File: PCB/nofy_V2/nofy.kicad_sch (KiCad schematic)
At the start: 153 parts, among them J18 PIn1x4, J21 PIn1x4, J32 PIn1x4, J33 PIn1x4, SW1 SW_SPDT, SW10 SW_PUSH, SW11 SW_PUSH, SW12 SW_PUSH, SW13 SW_PUSH, SW14 SW_PUSH, SW15 SW_PUSH, SW16 SW_PUSH, SW17 SW_PUSH, SW18 SW_PUSH, SW19 SW_PUSH, SW2 SW_SPDT, SW20 SW_PUSH, SW21 SW_PUSH, SW22 SW_PUSH, SW23 SW_PUSH, SW24 SW_PUSH, SW25 SW_PUSH, SW26 SW_PUSH, SW27 SW_PUSH, SW28 SW_PUSH, SW29 SW_PUSH, SW3 RotaryEncoder, SW30 SW_PUSH, SW31 SW_PUSH, SW32 SW_PUSH, SW33 SW_PUSH, SW34 SW_PUSH, SW35 SW_PUSH, SW36 SW_PUSH, SW37 SW_PUSH, SW38 SW_PUSH, SW39 SW_PUSH, SW4 RotaryEncoder, SW40 SW_PUSH, SW41 SW_PUSH, SW42 SW_PUSH, SW43 SW_PUSH, SW44 SW_PUSH, SW45 SW_PUSH, SW46 SW_PUSH, SW47 SW_PUSH, SW48 SW_PUSH, SW49 SW_PUSH, SW5 SW_PUSH, SW50 SW_PUSH, SW51 SW_PUSH, SW52 SW_PUSH, SW53 SW_PUSH, SW54 SW_PUSH, SW55 SW_PUSH, SW6 SW_PUSH, SW7 SW_PUSH, SW8 SW_PUSH, SW9 SW_PUSH

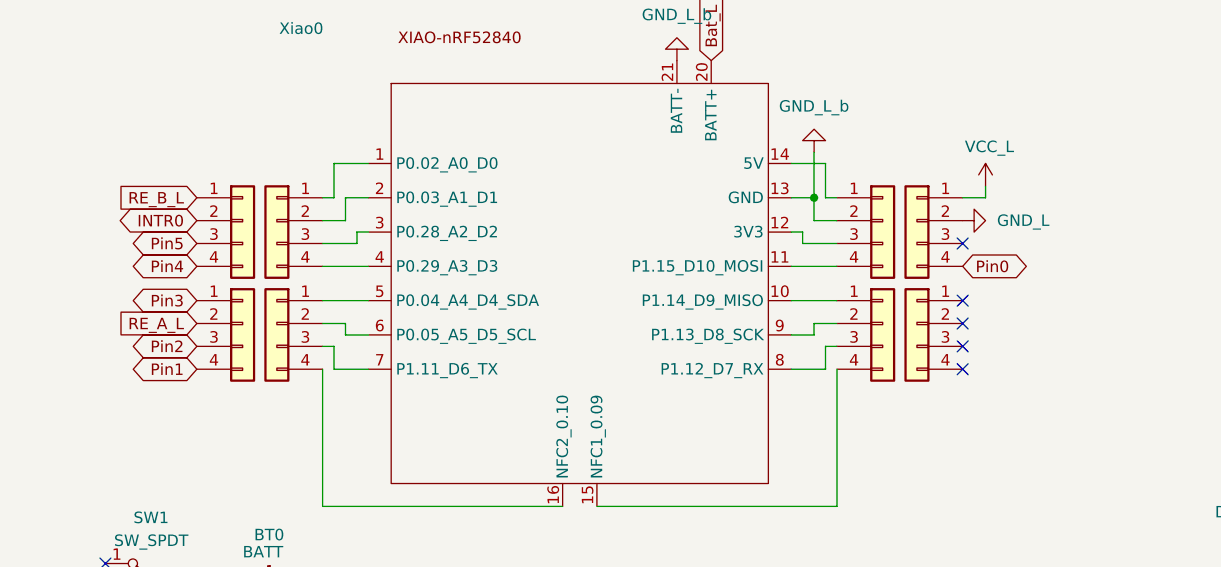
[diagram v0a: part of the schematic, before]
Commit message: PCB
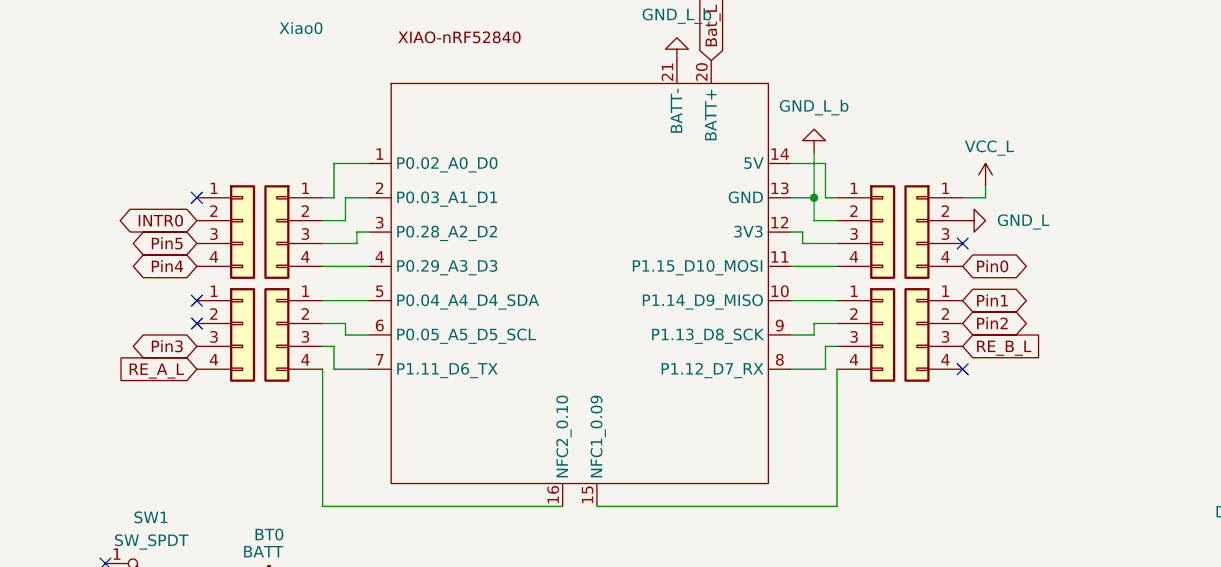
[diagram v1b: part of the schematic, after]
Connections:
- net Pin1: now also Con_L_6.1 (Pin_1); no longer Con_L_2.4 (Pin_4)
- net Pin2: now also Con_L_6.2 (Pin_2); no longer Con_L_2.3 (Pin_3)
- net Pin3: now also Con_L_2.3 (Pin_3); no longer Con_L_2.1 (Pin_1)
- net RE_A_L: now also Con_L_2.4 (Pin_4); no longer Con_L_2.2 (Pin_2)
- net RE_B_L: now also Con_L_6.3 (Pin_3); no longer Con_L_0.1 (Pin_1)
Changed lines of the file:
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@@
 	)
 	(no_connect
-		(at 114.3 55.88)
-	)
-	(no_connect
 		(at 19.05 82.55)
 	)
@@
 	)
 	(no_connect
-		(at 114.3 53.34)
+		(at 29.21 55.88)
 	)
 	(no_connect
-		(at 114.3 58.42)
+		(at 29.21 41.91)
+	)
+	(no_connect
+		(at 29.21 53.34)
 	)
 	(wire
@@
 		)
 	)
+	(global_label "Pin2"
+		(shape bidirectional)
+		(at 114.3 55.88 0)
+		(fields_autoplaced yes)
+		(effects
+			(font
+				(size 1.27 1.27)
+			)
+			(justify left)
+		)
+		(property "Intersheetrefs" "${INTERSHEET_REFS}"
+			(at 122.6298 55.88 0)
+			(effects
+				(font
+					(size 1.27 1.27)
+				)
+				(justify left)
+				(hide yes)
+			)
+		)
+	)
 	(global_label "Pin4"
 		(shape bidirectional)
@@
 		)
 	)
-	(global_label "Pin2"
-		(shape bidirectional)
-		(at 29.21 58.42 180)
-		(fields_autoplaced yes)
-		(effects
-			(font
-				(size 1.27 1.27)
-			)
-			(justify right)
-		)
-		(property "Intersheetrefs" "${INTERSHEET_REFS}"
-			(at 20.8802 58.42 0)
-			(effects
-				(font
-					(size 1.27 1.27)
-				)
-				(justify right)
-				(hide yes)
-			)
-		)
-	)
 	(global_label "RE_B_R"
 		(shape input)
@@
 		)
 	)
-	(global_label "Pin1"
-		(shape bidirectional)
-		(at 29.21 60.96 180)
+	(global_label "RE_B_L"
+		(shape input)
+		(at 114.3 58.42 0)
 		(fields_autoplaced yes)
 		(effects
@@
 				(size 1.27 1.27)
 			)
-			(justify right)
+			(justify left)
 		)
 		(property "Intersheetrefs" "${INTERSHEET_REFS}"
-			(at 20.8802 60.96 0)
+			(at 123.9375 58.42 0)
 			(effects
 				(font
 					(size 1.27 1.27)
 				)
-				(justify right)
+				(justify left)
 				(hide yes)
 			)
@@
 		)
 	)
-	(global_label "RE_A_L"
-		(shape input)
-		(at 29.21 55.88 180)
-		(fields_autoplaced yes)
-		(effects
-			(font
-				(size 1.27 1.27)
-			)
-			(justify right)
-		)
-		(property "Intersheetrefs" "${INTERSHEET_REFS}"
-			(at 19.7539 55.88 0)
-			(effects
-				(font
-					(size 1.27 1.27)
-				)
-				(justify right)
-				(hide yes)
-			)
-		)
-	)
 	(global_label "INTR0"
 		(shape bidirectional)
@@
 		)
 	)
+	(global_label "RE_A_L"
+		(shape input)
+		(at 29.21 60.96 180)
+		(fields_autoplaced yes)
+		(effects
+			(font
+				(size 1.27 1.27)
+			)
+			(justify right)
+		)
+		(property "Intersheetrefs" "${INTERSHEET_REFS}"
+			(at 19.7539 60.96 0)
+			(effects
+				(font
+					(size 1.27 1.27)
+				)
+				(justify right)
+				(hide yes)
+			)
+		)
+	)
 	(global_label "RE_B_L"
 		(shape input)
@@
 		)
 	)
+	(global_label "Pin1"
+		(shape bidirectional)
+		(at 114.3 53.34 0)
+		(fields_autoplaced yes)
+		(effects
+			(font
+				(size 1.27 1.27)
+			)
+			(justify left)
+		)
+		(property "Intersheetrefs" "${INTERSHEET_REFS}"
+			(at 122.6298 53.34 0)
+			(effects
+				(font
+					(size 1.27 1.27)
+				)
+				(justify left)
+				(hide yes)
+			)
+		)
+	)
 	(global_label "SCLK"
 		(shape input)
@@
 		)
 	)
-	(global_label "INTR1"
+	(global_label "Pin3"
 		(shape bidirectional)
-		(at 22.86 200.66 180)
+		(at 29.21 58.42 180)
 		(fields_autoplaced yes)
 		(effects
@@
 		)
 		(property "Intersheetrefs" "${INTERSHEET_REFS}"
-			(at 13.3811 200.66 0)
+			(at 20.8802 58.42 0)
 			(effects
 				(font
@@
 		)
 	)
-	(global_label "Pin3"
+	(global_label "INTR1"
 		(shape bidirectional)
-		(at 29.21 53.34 180)
+		(at 22.86 200.66 180)
 		(fields_autoplaced yes)
 		(effects
@@
 		)
 		(property "Intersheetrefs" "${INTERSHEET_REFS}"
-			(at 20.8802 53.34 0)
+			(at 13.3811 200.66 0)
 			(effects
 				(font
@@
 				(hide yes)
 			)
-		)
-	)
-	(global_label "RE_B_L"
-		(shape input)
-		(at 29.21 41.91 180)
-		(fields_autoplaced yes)
-		(effects
-			(font
-				(size 1.27 1.27)
-			)
-			(justify right)
-		)
-		(property "Intersheetrefs" "${INTERSHEET_REFS}"
-			(at 19.5725 41.91 0)
-			(effects
-				(font
-					(size 1.27 1.27)
-				)
-				(justify right)
-				(hide yes)
-			)

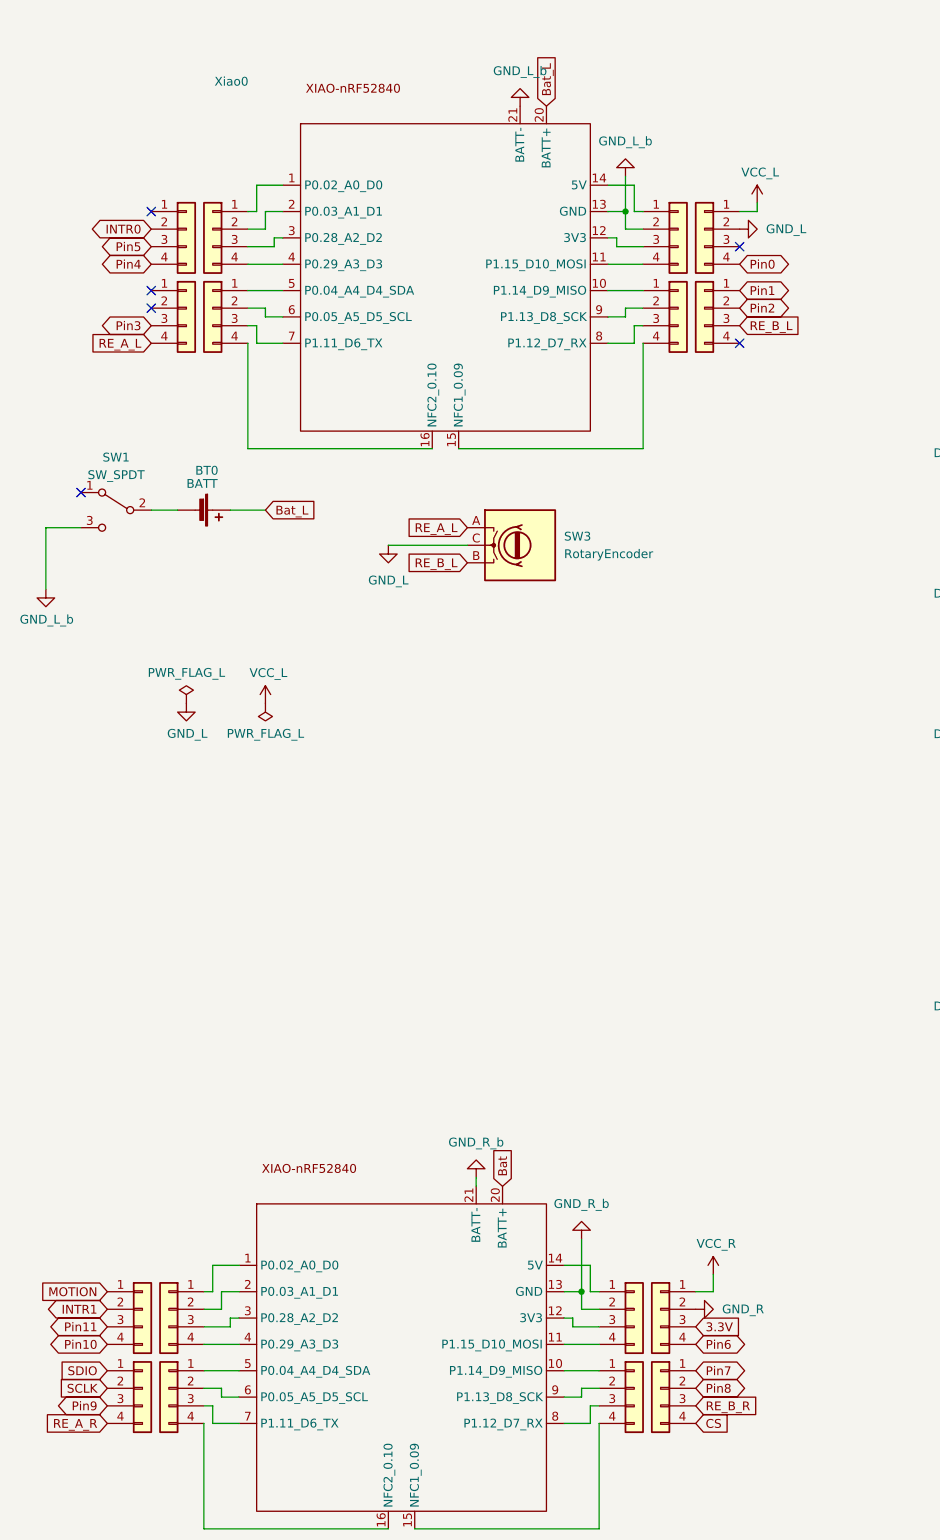
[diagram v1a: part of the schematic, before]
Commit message: pcb
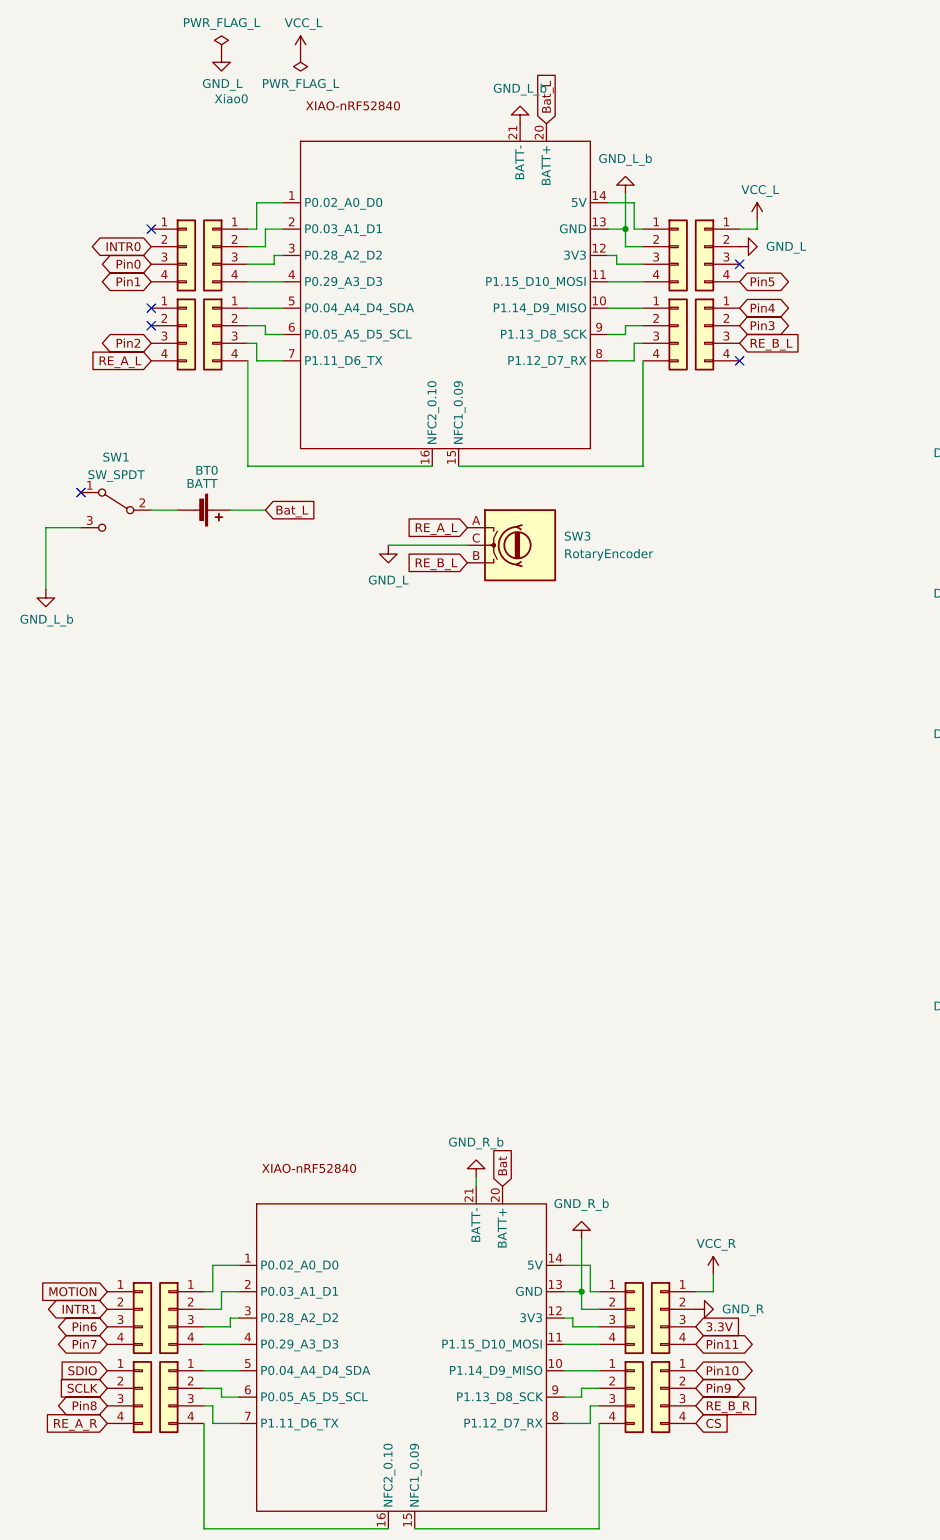
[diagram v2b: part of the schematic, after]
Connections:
- net Pin0: now also Con_L_0.3 (Pin_3); no longer Con_L_4.4 (Pin_4)
- net Pin1: now also Con_L_0.4 (Pin_4); no longer Con_L_6.1 (Pin_1)
- net Pin10: now also Con_L_14.1 (Pin_1); no longer Con_L_8.4 (Pin_4)
- net Pin11: now also Con_L_12.4 (Pin_4); no longer Con_L_8.3 (Pin_3)
- net Pin2: now also Con_L_2.3 (Pin_3); no longer Con_L_6.2 (Pin_2)
- net Pin3: now also Con_L_6.2 (Pin_2); no longer Con_L_2.3 (Pin_3)
- net Pin4: now also Con_L_6.1 (Pin_1); no longer Con_L_0.4 (Pin_4)
- net Pin5: now also Con_L_4.4 (Pin_4); no longer Con_L_0.3 (Pin_3)
- net Pin6: now also Con_L_8.3 (Pin_3); no longer Con_L_12.4 (Pin_4)
- net Pin7: now also Con_L_8.4 (Pin_4); no longer Con_L_14.1 (Pin_1)
- net Pin8: now also Con_L_10.3 (Pin_3); no longer Con_L_14.2 (Pin_2)
- net Pin9: now also Con_L_14.2 (Pin_2); no longer Con_L_10.3 (Pin_3)
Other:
- moved on the sheet: Xiao0
